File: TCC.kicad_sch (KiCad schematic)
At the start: 4 parts, among them IC1 FSBB30CH60

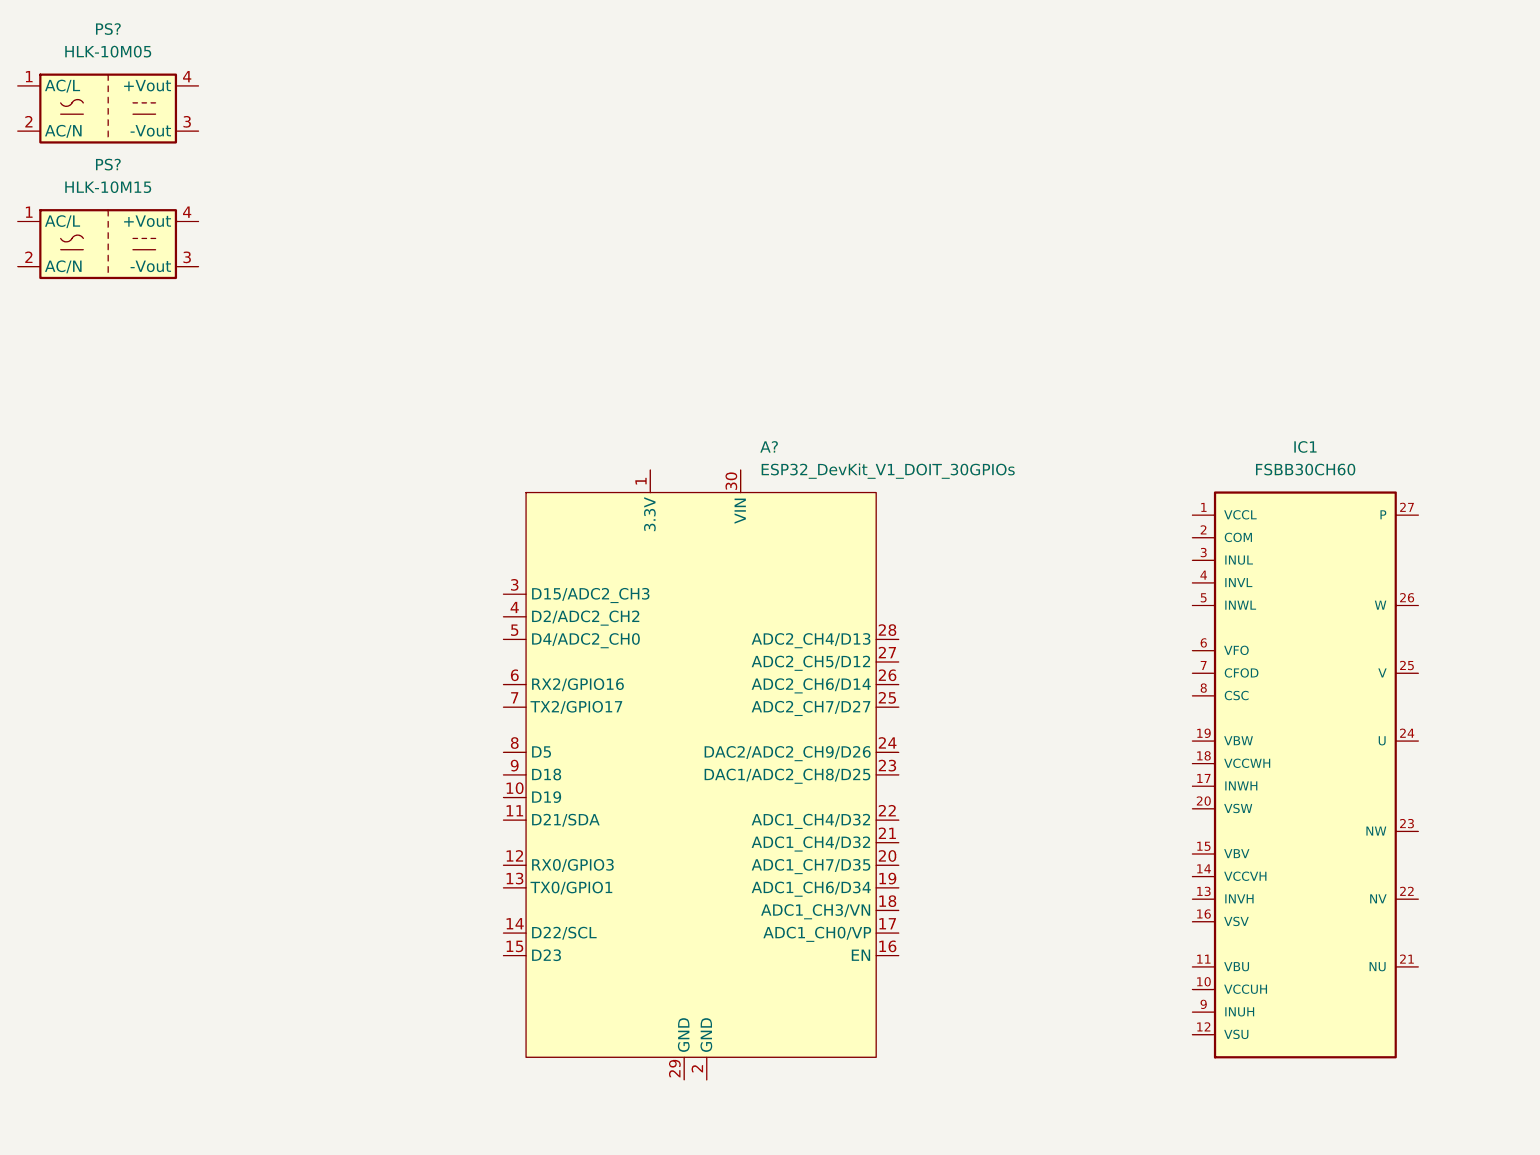
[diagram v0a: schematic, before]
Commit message: Init
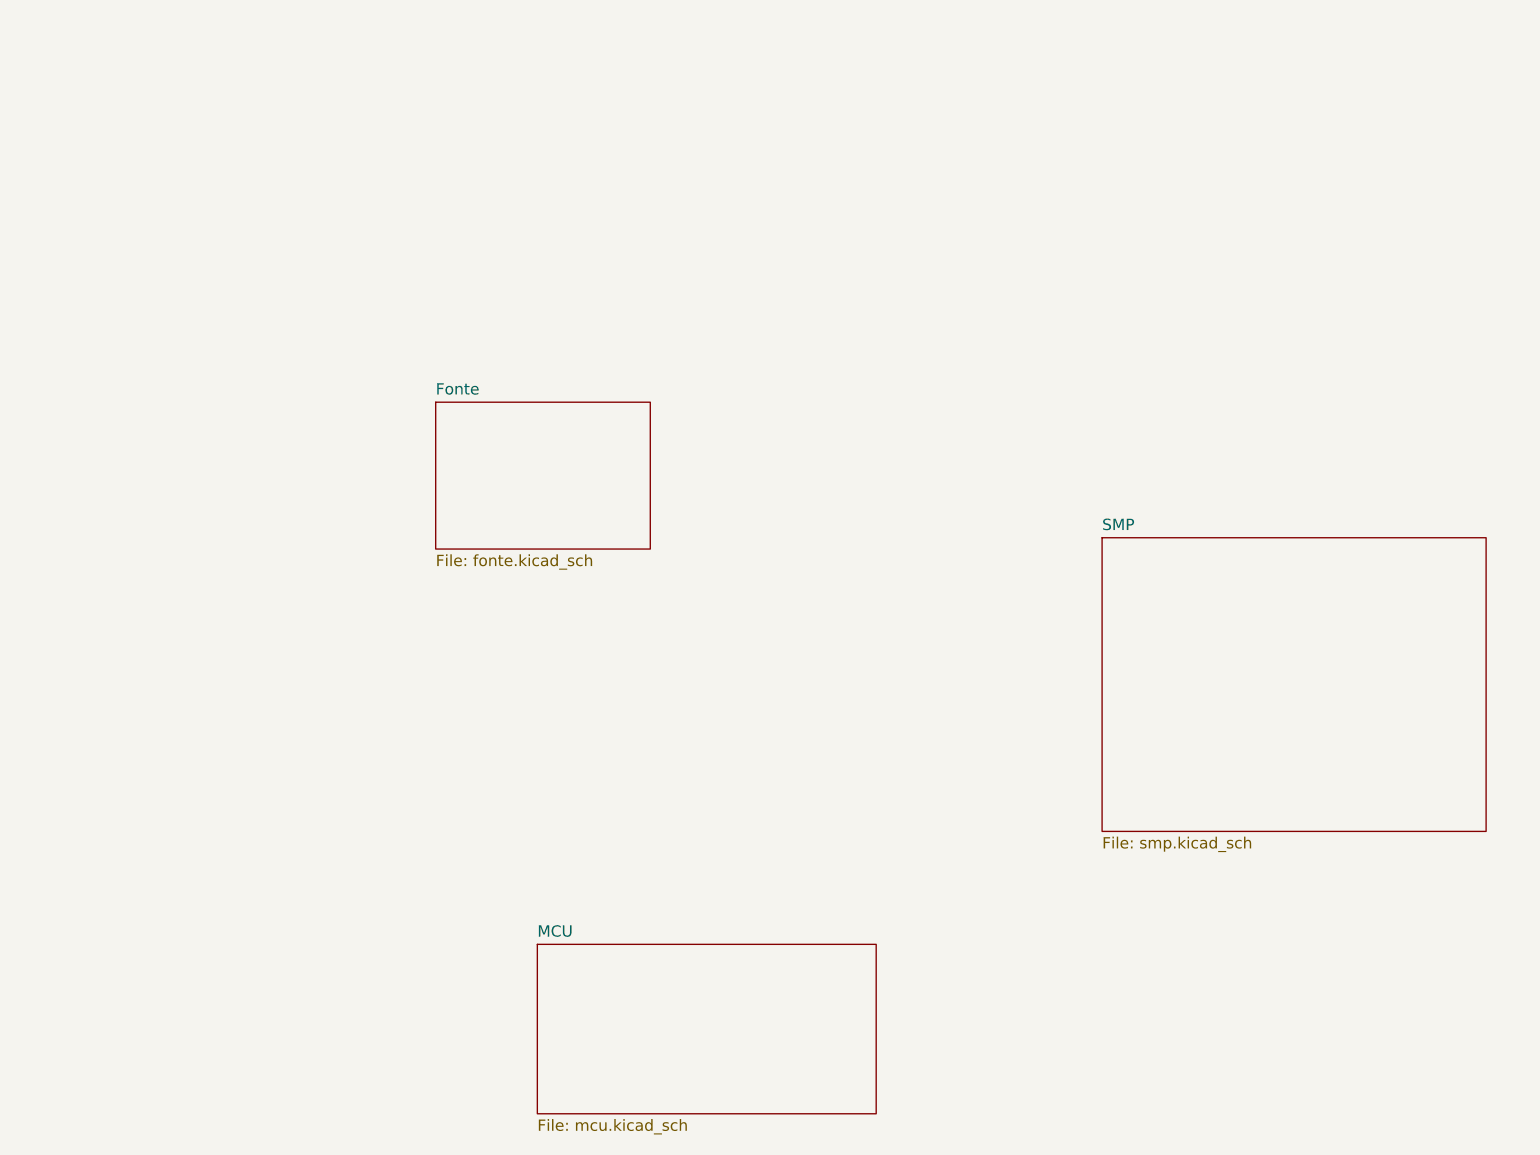
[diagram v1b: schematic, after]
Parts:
- removed A?: ESP32_DevKit_V1_DOIT_30GPIOs, PCM_SL_Development_Boards:DOIT_ESP32_DEVKIT_30Pins, symbol PCM_SL_Development_Board:ESP32_DevKit_V1_DOIT_30GPIOs
- removed IC1: FSBB30CH60, FSBB30CH60:FSBB30CH60, symbol FSBB30CH60:FSBB30CH60
- removed PS?: HLK-10M15, Converter_ACDC:Converter_ACDC_Hi-Link_HLK-10Mxx, symbol Converter_ACDC:HLK-10M15
- removed PS?: HLK-10M05, Converter_ACDC:Converter_ACDC_Hi-Link_HLK-10Mxx, symbol Converter_ACDC:HLK-10M05
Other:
- added sheet Fonte (fonte.kicad_sch)
- added sheet MCU (mcu.kicad_sch)
- added sheet SMP (smp.kicad_sch)
- company: (none) -> UFPEL
- title: (none) -> Inversor de Bancada

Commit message: midsave
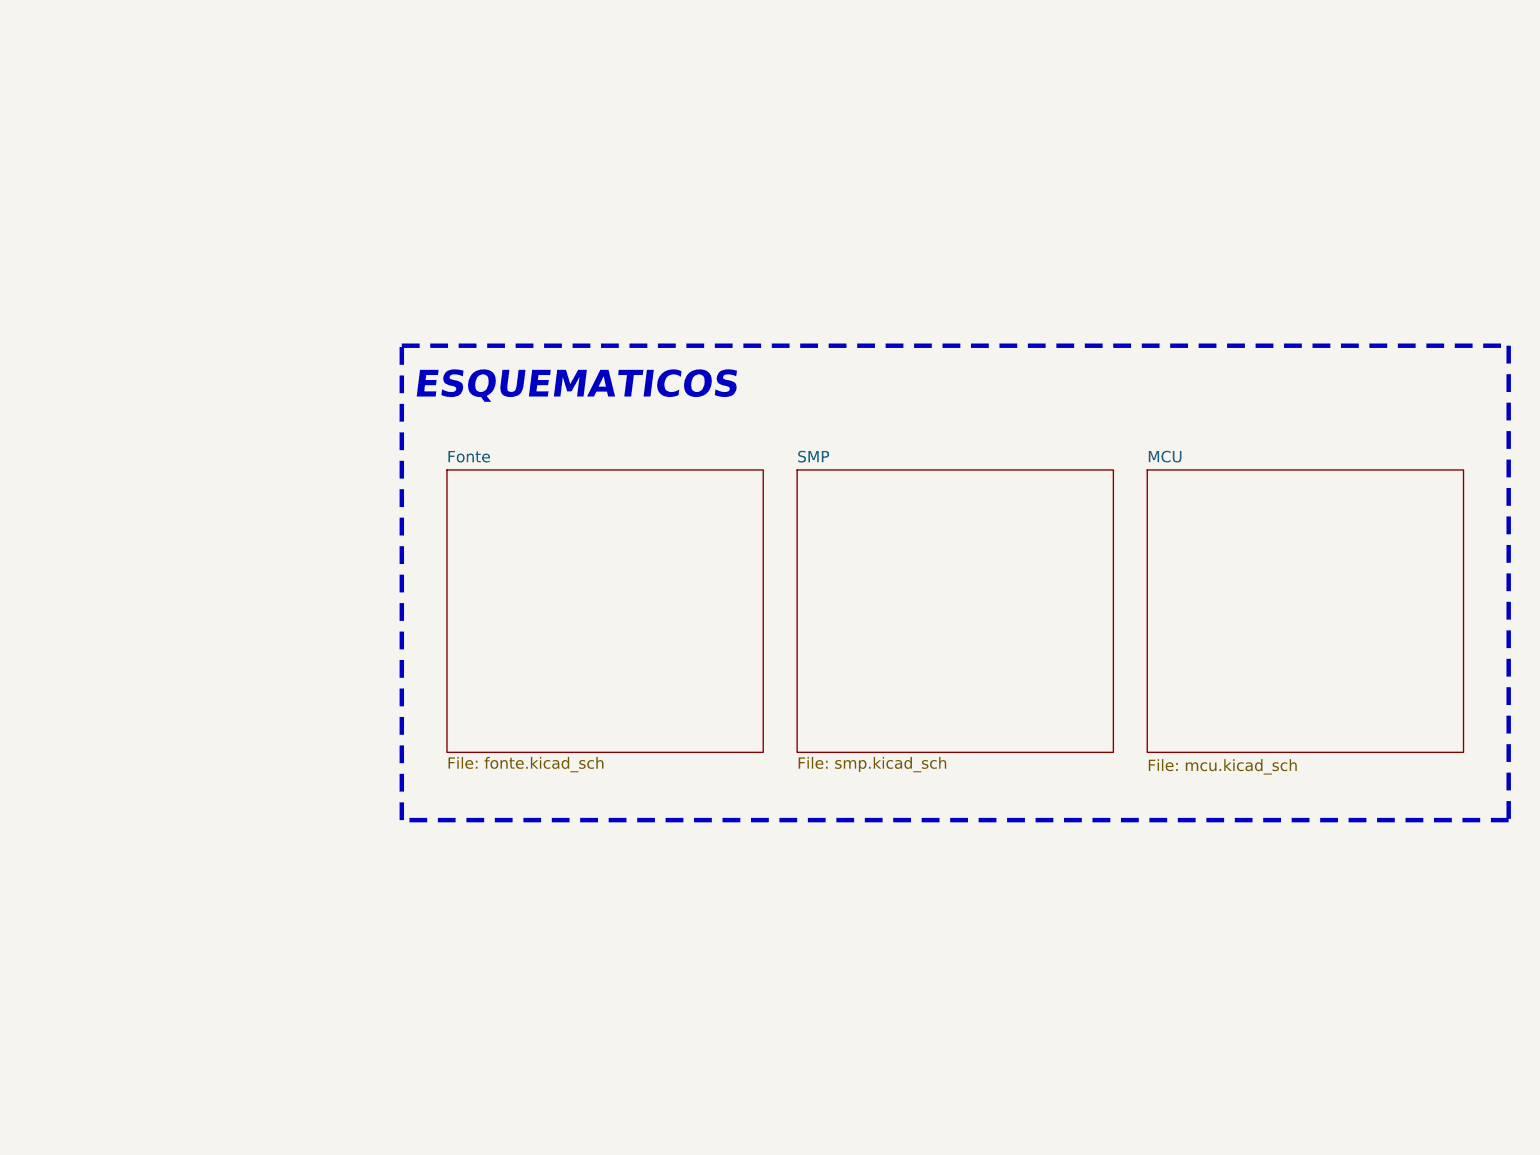
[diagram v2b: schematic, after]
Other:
- note added: "ESQUEMATICOS"
- company: UFPEL -> Autor: José Fonseca

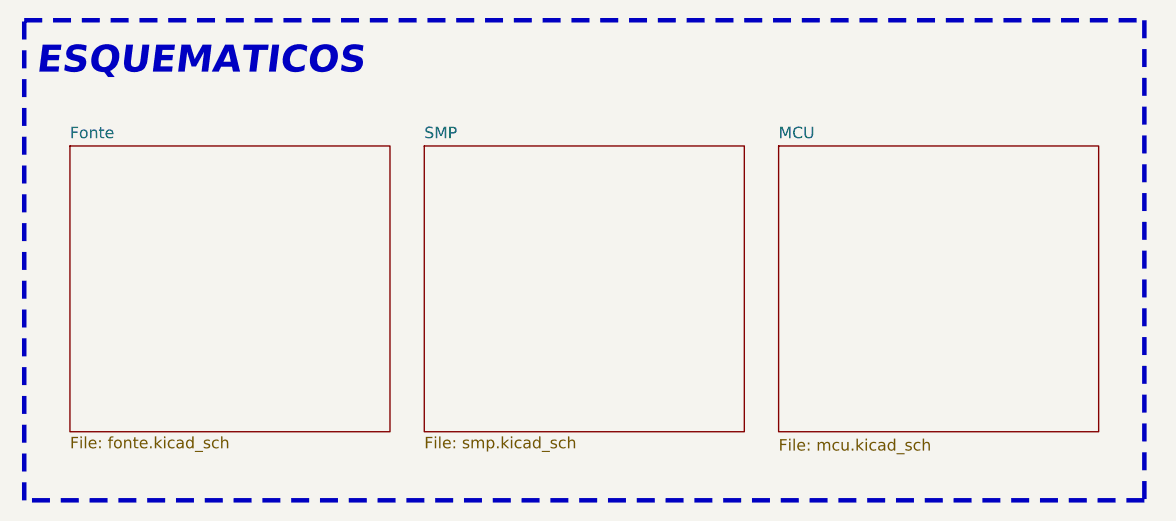
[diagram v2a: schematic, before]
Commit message: f
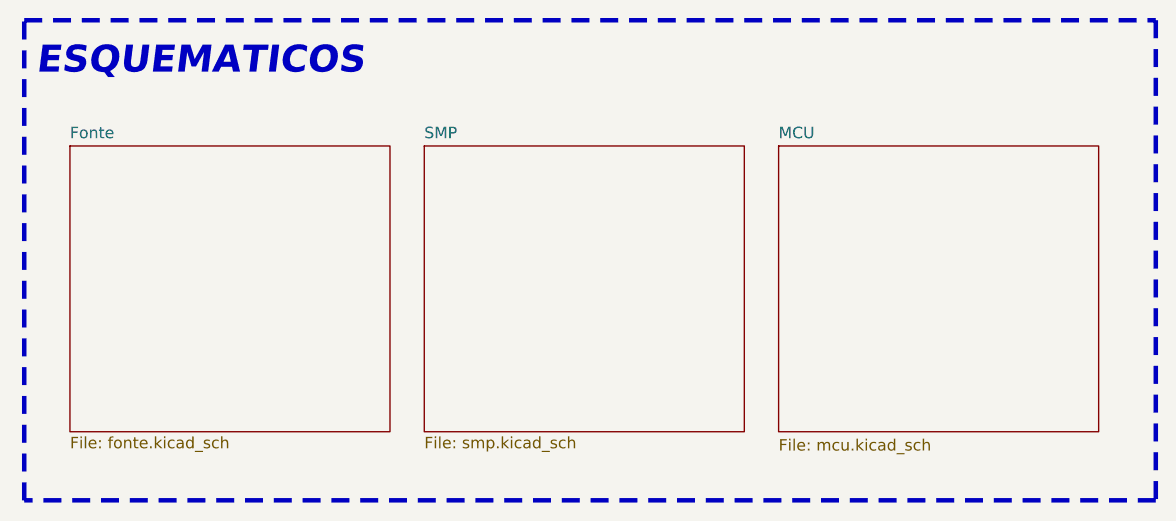
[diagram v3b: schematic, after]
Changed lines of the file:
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@@
 	(rectangle
 		(start 80.01 63.5)
-		(end 204.47 116.84)
+		(end 205.74 116.84)
 		(stroke
 			(width 0.5)
